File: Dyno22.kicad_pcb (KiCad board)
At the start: 2 copper layers, 57 parts, among them J1 Pwr Input, J2 Display, J3 Pwr Output, J4 BPM & Sensors, J7 UART, SW1 SW_DPST_x2, U1 TS2937CW50, U2 LM324, U3 Demux

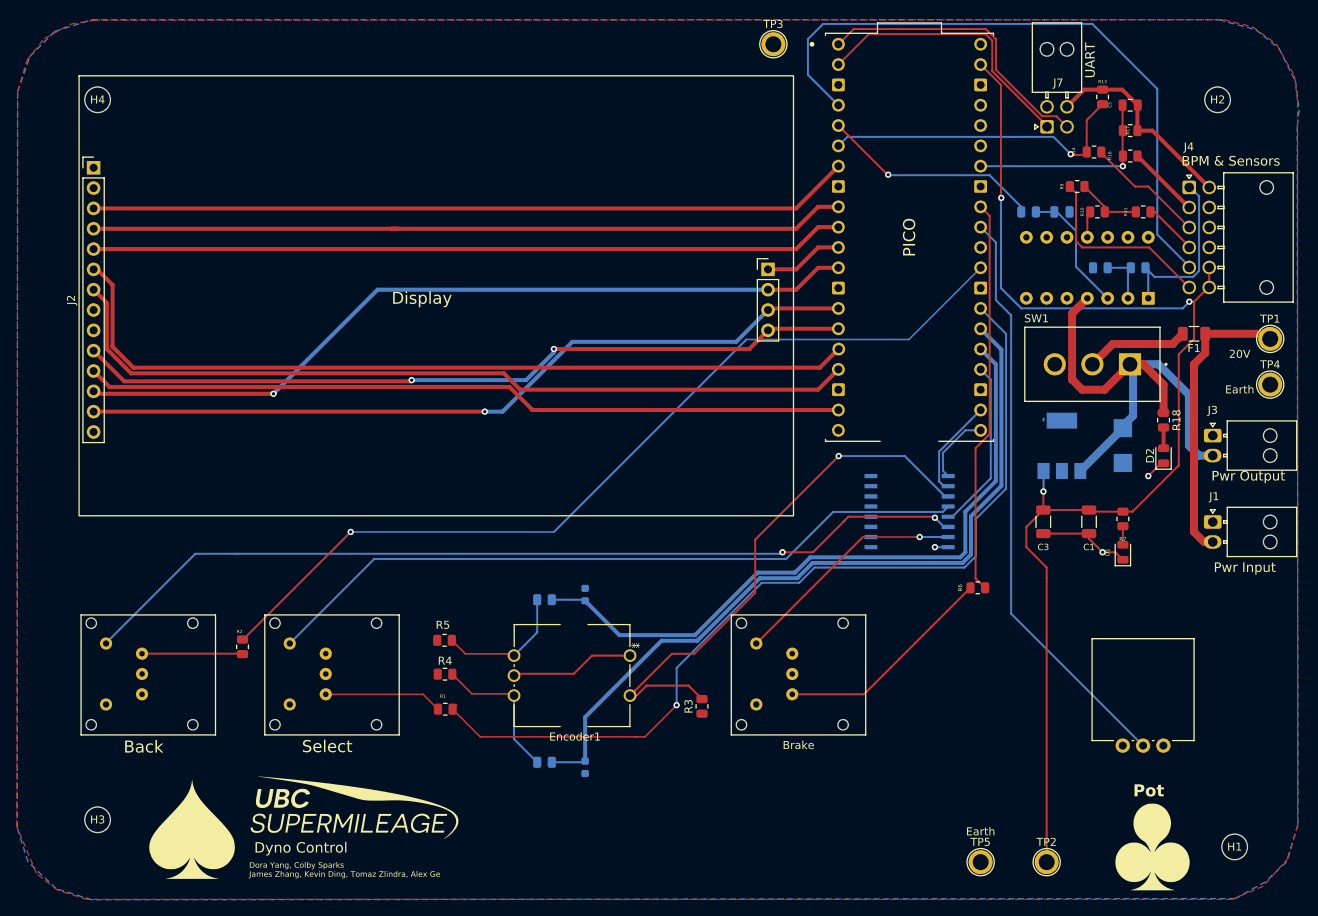
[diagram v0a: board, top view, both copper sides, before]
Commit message: v2
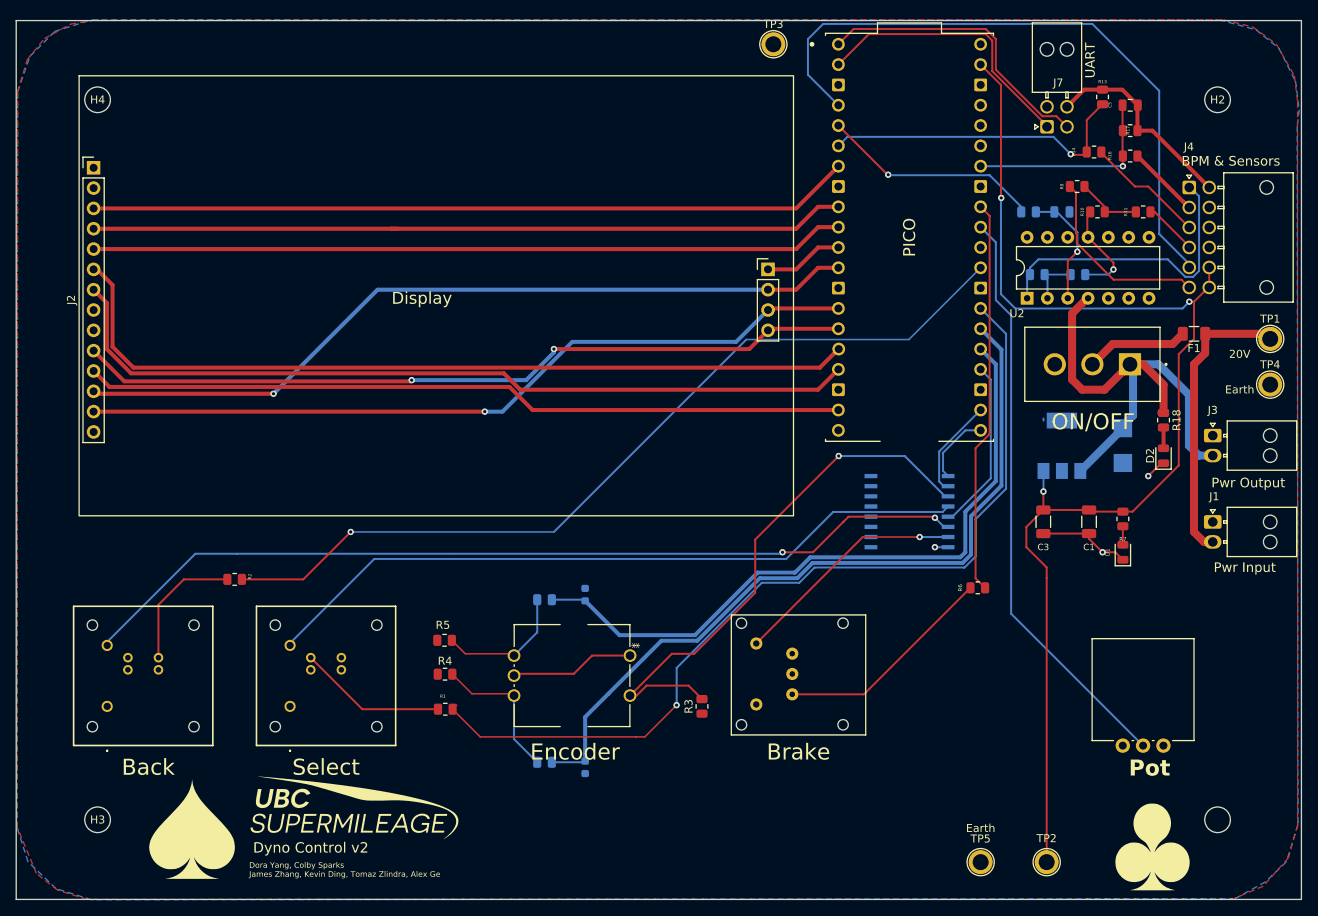
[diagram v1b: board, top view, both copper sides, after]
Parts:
- Back: renamed from S1; footprint LP11EE1NCSYG:LP11EE1NCSYG -> KP0115ANBKG03RGBP3SJB:KP0115ANBKG03RGBP3SJB
- R4, R5: value 10kΩ -> 1kΩ
- Select: renamed from S2; footprint LP11EE1NCSYG:LP11EE1NCSYG -> KP0115ANBKG03RGBP3SJB:KP0115ANBKG03RGBP3SJB
- U2: moved to F.Cu
- moved U2 15.1 mm to (188.7, 67.3)
- moved R15 12.6 mm to (190.0, 64.3), turned to 180 degrees
- moved Back 11.9 mm to (73.7, 118.3), turned to 90 degrees
- moved Select 11.9 mm to (96.6, 118.3), turned to 90 degrees
- moved R2 8.49 mm to (89.6, 102.5), turned to 0 degrees
- moved H1 4.00 mm to (212.5, 132.5)
- moved R12 2.93 mm to (195.0, 64.3), turned to 0 degrees
- renumbered Encoder1 to Encoder, SW1 to ON/OFF
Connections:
- Back pad 2: /BTN_BACK -> +3.3V
- R1 pad 1: Net-(S2-L1_Y) -> Net-(S2-K_B)
- R2 pad 1: Net-(S1-L2_G) -> Net-(S1-K_R)
- Select pad 2: /BTN_SELECT -> +3.3V
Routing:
- net Net-(S2-K_B): track 0.00 -> 18.6 mm
- net Net-(S1-K_R): track 0.00 -> 16.5 mm
- net /BPM_CTRL: track 22.5 -> 37.8 mm
- net Net-(S2-L1_Y): track 14.8 -> 0.00 mm
- net Net-(S1-L2_G): track 12.6 -> 0.00 mm
- net Earth: track 59.5 -> 68.7 mm, vias 2 -> 3
- net /LED_BACK: track 111.5 -> 108.5 mm
- net Net-(U2-+): track 16.0 -> 15.0 mm, vias 0 -> 1
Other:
- board outline added: 160.7 x 109.9 mm
- board text added: "Dyno Control v2"
- board text removed: "Dyno Control"
